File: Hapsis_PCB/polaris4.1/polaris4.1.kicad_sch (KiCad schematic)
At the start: 94 parts, among them J1 Screw_Terminal_01x02, J10 SD CARD, J11 Screw_Terminal_01x02, J12 Screw_Terminal_01x02, J13 Screw_Terminal_01x02, J2 Screw_Terminal_01x02, J3 Screw_Terminal_01x02, J4 Screw_Terminal_01x02, J5 Screw_Terminal_01x02, J6 Screw_Terminal_01x02, J7 Screw_Terminal_01x02, J8 BARO, J9 Pyro Safety Switch Terminal, Q1 NTR4501NT1G, Q2 NTR4501NT1G, Q3 NTR4501NT1G, Q4 NTR4501NT1G, Q5 NTR4501NT1G, Q6 NTR4501NT1G, Q7 NTR4501NT1G, Q8 NTR4501NT1G, U2 TPS56339DDC

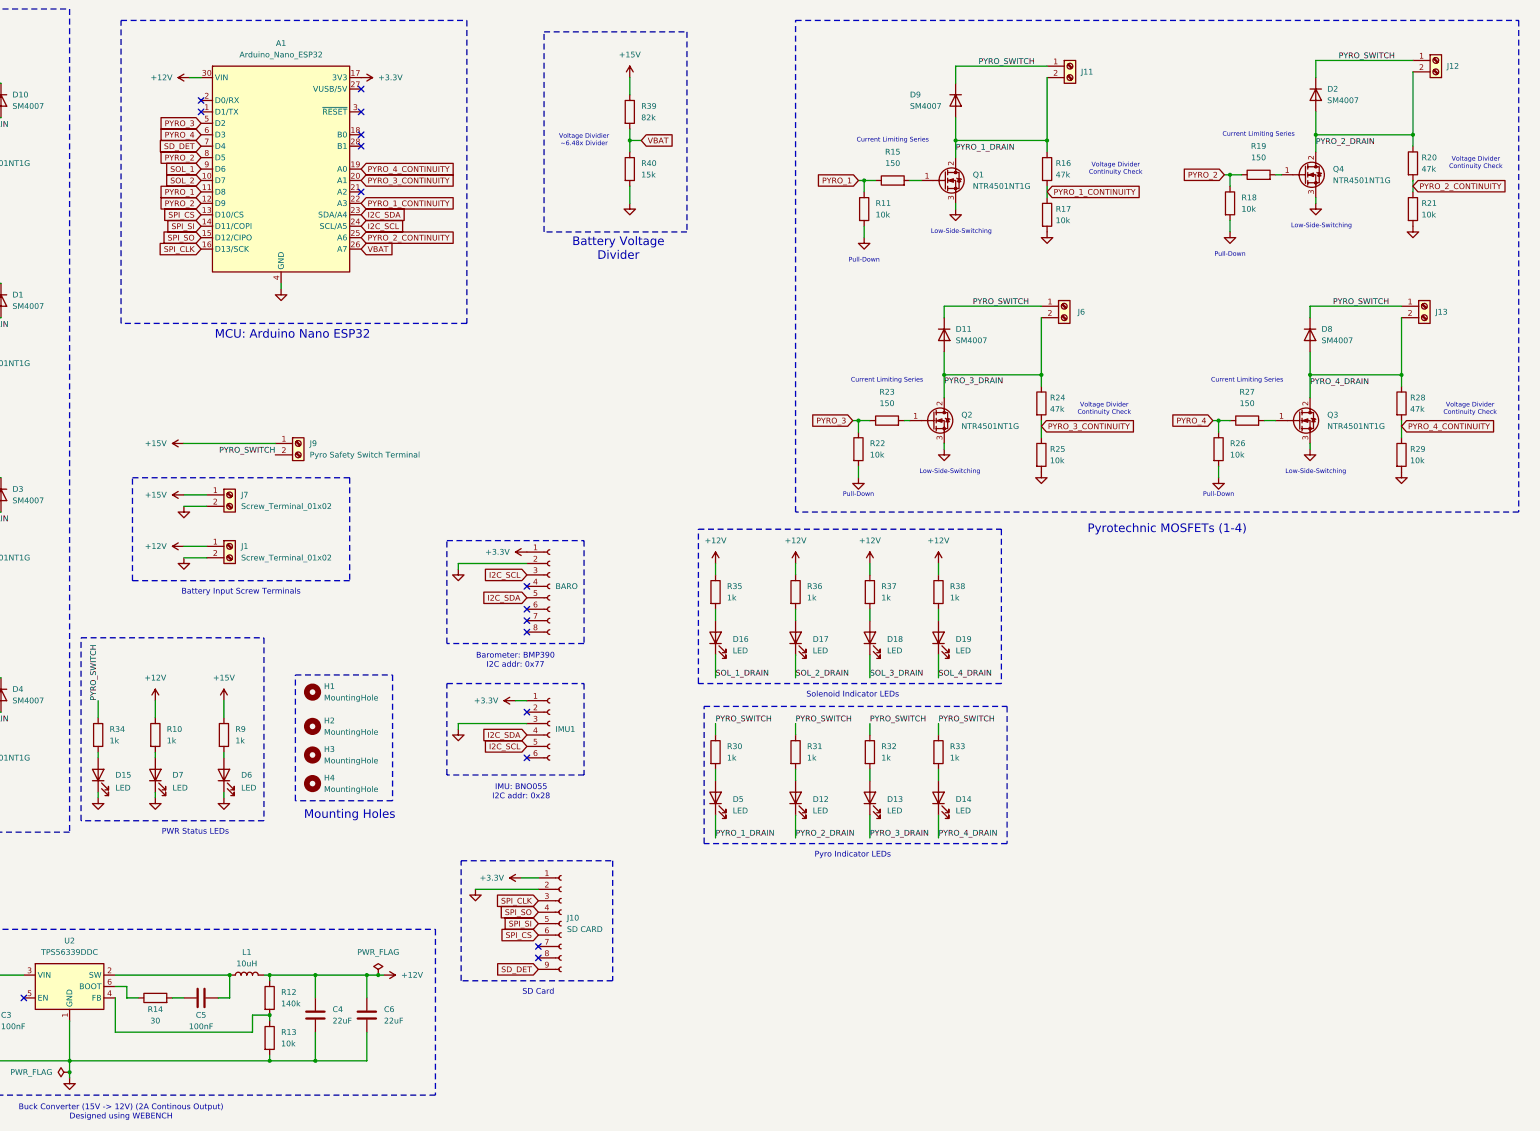
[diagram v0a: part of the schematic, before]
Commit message: updated PCB
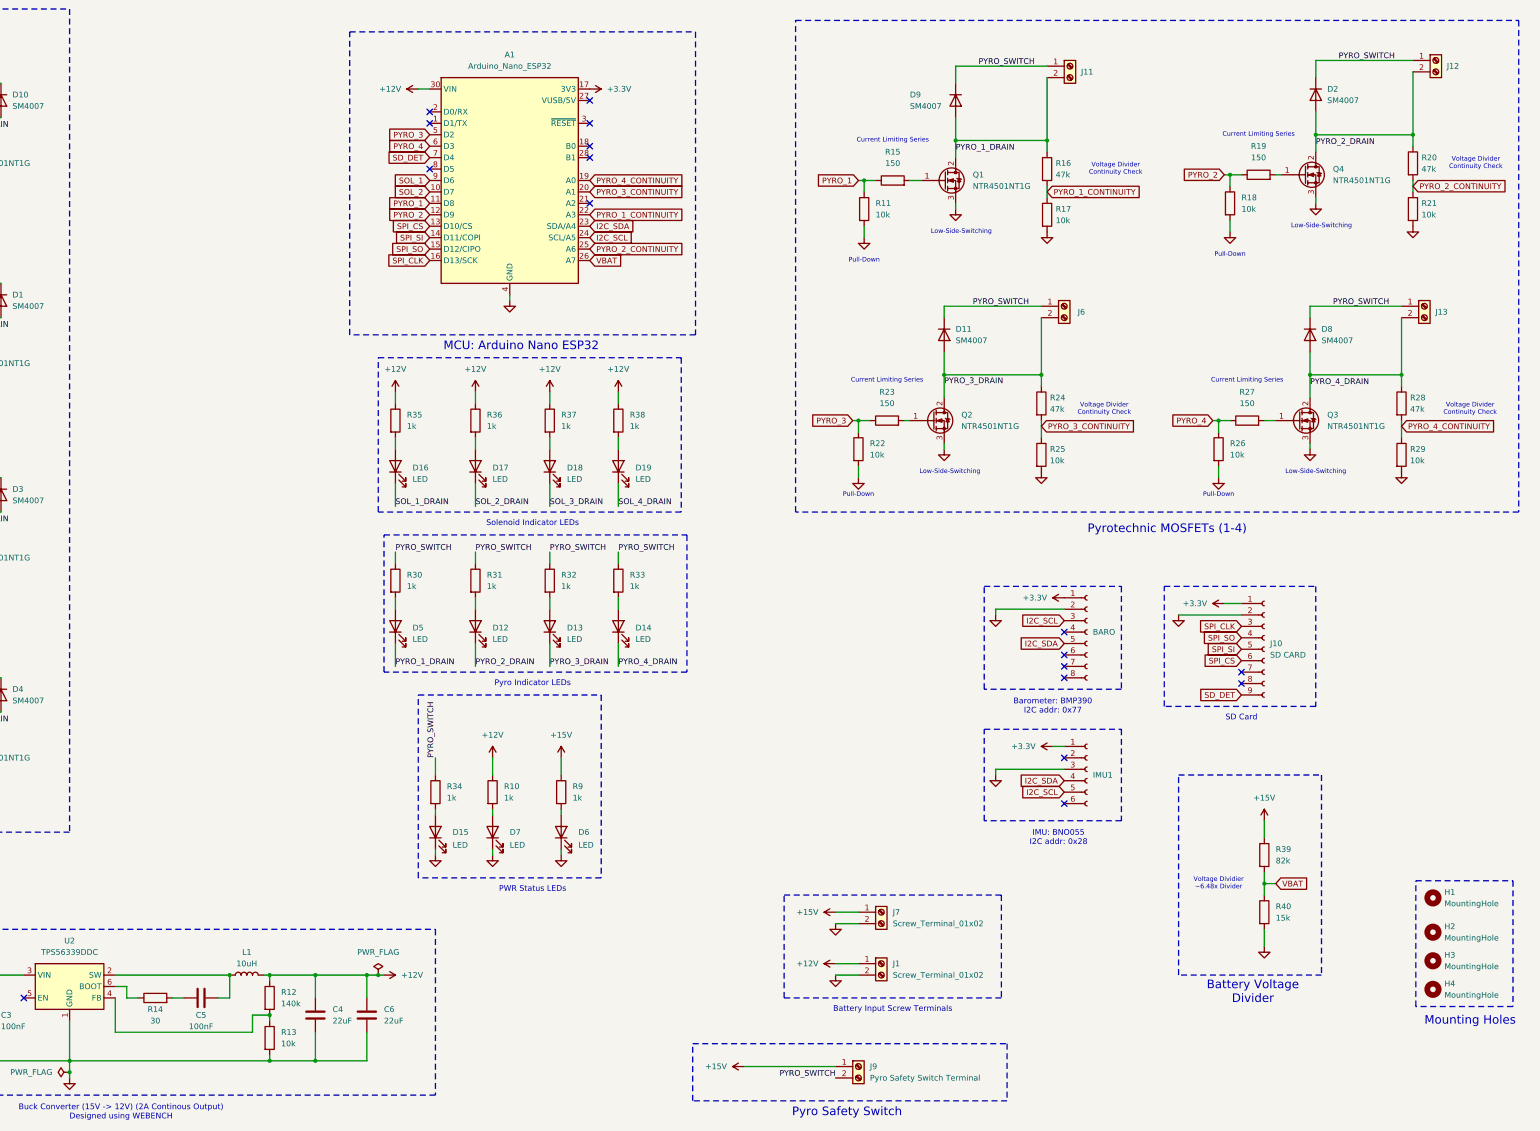
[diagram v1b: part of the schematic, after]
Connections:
- net PYRO_2: no longer A1.8 (D5)
- no-connect marks 16 -> 17
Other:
- note added: "Pyro Safety Switch"
- moved on the sheet: A1, D12, D13, D14, D15, D16, D17, D18, D19, D5, D6, D7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
